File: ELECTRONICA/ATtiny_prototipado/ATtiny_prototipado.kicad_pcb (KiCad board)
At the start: 2 copper layers, 21.4 x 26.4 mm, 5 parts, among them J1 Conector_izquierdo, J2 Conector_derecho, U1 ATtiny1634-SU

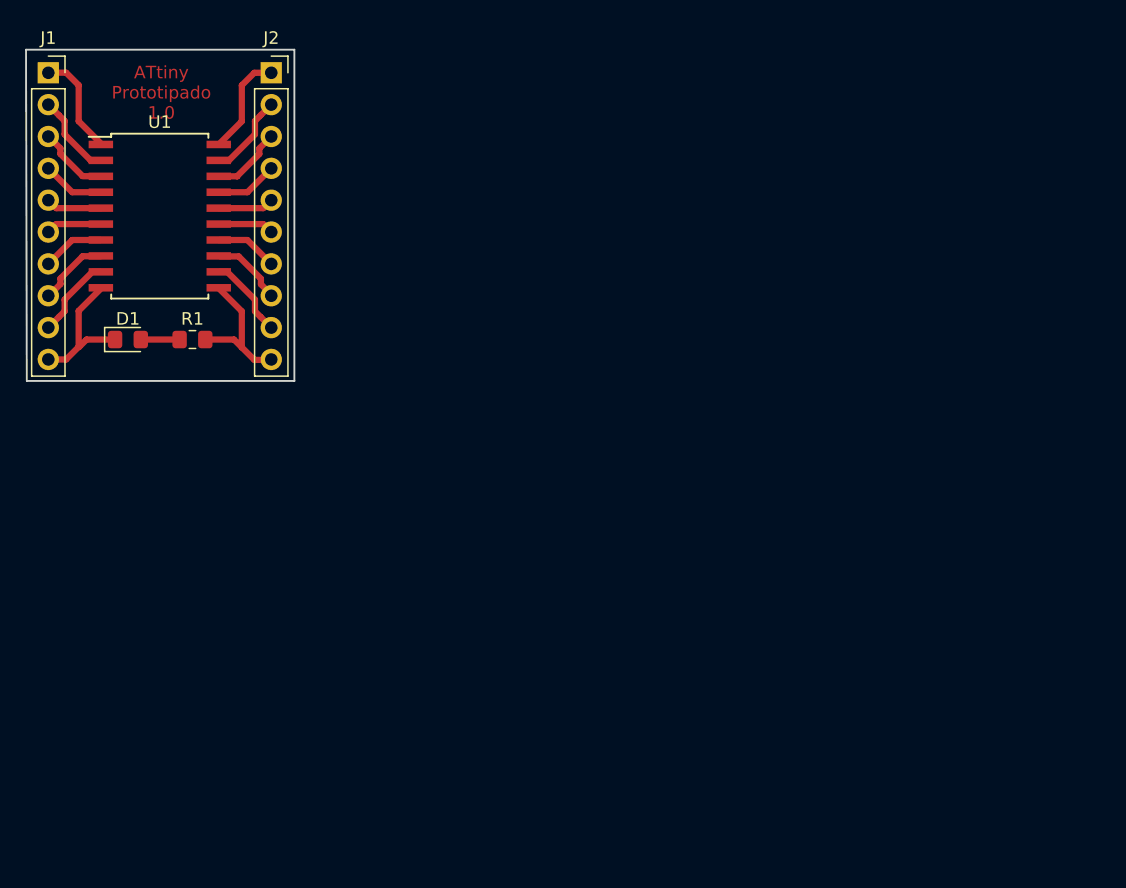
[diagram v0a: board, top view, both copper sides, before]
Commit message: 4-6-19
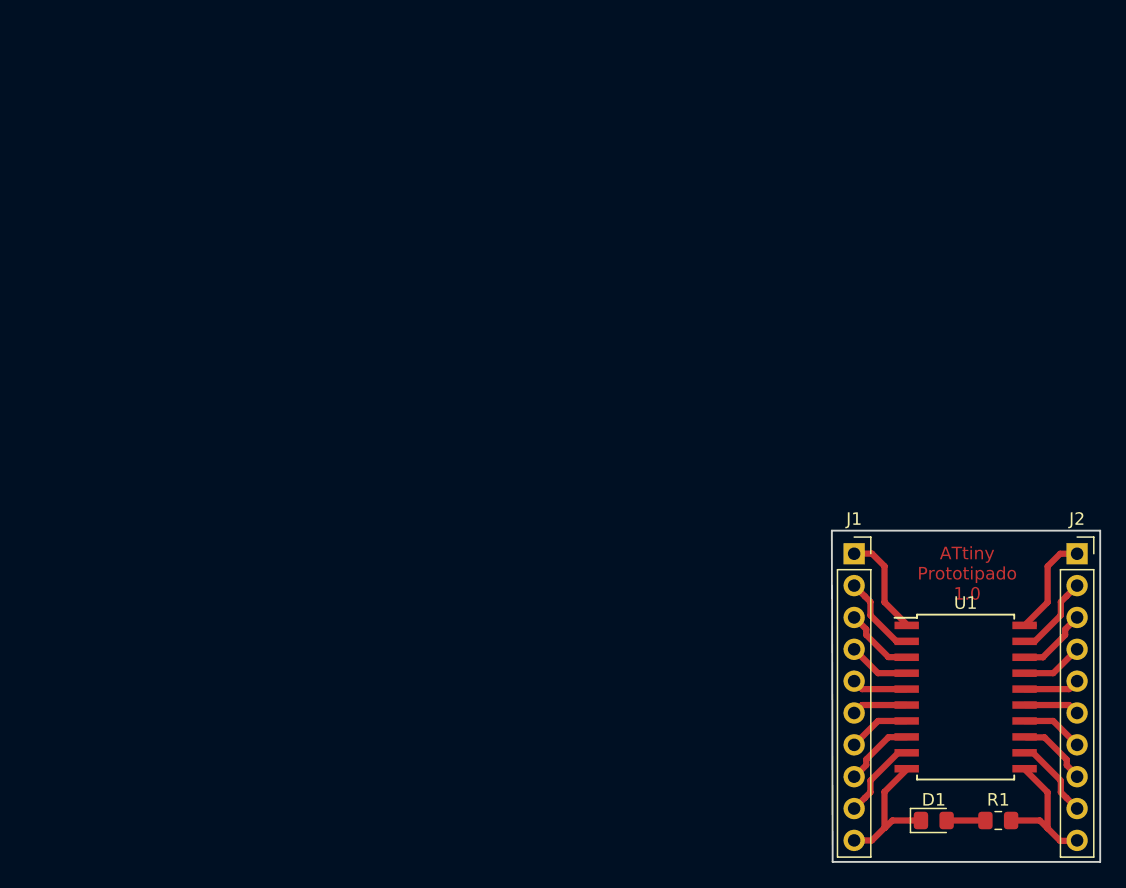
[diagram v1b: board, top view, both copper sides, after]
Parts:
- moved D1 74.8 mm to (103.0, 87.2)
- moved J1 74.8 mm to (96.6, 66.0)
- moved J2 74.8 mm to (114.4, 66.0)
- moved R1 74.8 mm to (108.1, 87.2)
- moved U1 74.8 mm to (105.5, 77.4)
